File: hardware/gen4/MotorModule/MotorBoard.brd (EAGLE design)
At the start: 34 x 61.7 mm, 67 parts, among them IC1 XMEGA16A4A, M1O1 TEST_PT, M1O2 TEST_PT, M1O3 TEST_PT

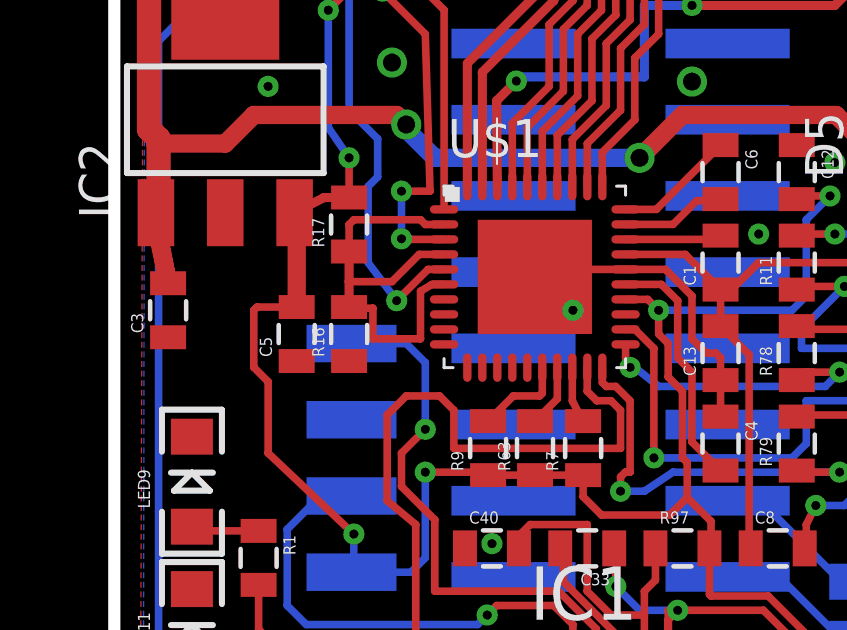
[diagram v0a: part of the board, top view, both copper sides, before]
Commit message: passes erc
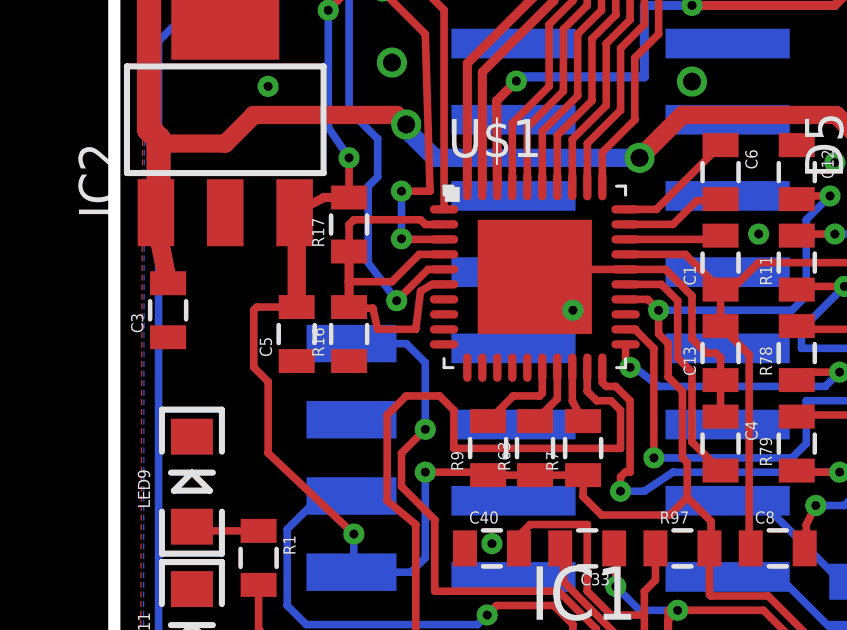
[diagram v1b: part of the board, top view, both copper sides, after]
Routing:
- net N$22: track 15.7 -> 14.8 mm
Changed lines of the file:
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@@
 <wire x1="9.9925" y1="10.06875" x2="9.5925" y2="10.06875" width="0.254" layer="1"/>
 <wire x1="9.5925" y1="10.06875" x2="9.2075" y2="9.8425" width="0.254" layer="1"/>
-<wire x1="9.2075" y1="9.8425" x2="9.2075" y2="8.255" width="0.254" layer="1"/>
-<wire x1="9.2075" y1="8.255" x2="7.62" y2="8.255" width="0.254" layer="1"/>
-<wire x1="7.62" y1="8.255" x2="7.62" y2="9.275" width="0.254" layer="1"/>
+<wire x1="9.2075" y1="9.8425" x2="9.04875" y2="8.5725" width="0.254" layer="1"/>
+<wire x1="9.04875" y1="8.5725" x2="7.77875" y2="8.5725" width="0.254" layer="1"/>
+<wire x1="7.77875" y1="8.5725" x2="7.62" y2="9.275" width="0.254" layer="1"/>
 <wire x1="9.9925" y1="12.06875" x2="9.36625" y2="12.065" width="0.254" layer="1"/>
 <wire x1="9.36625" y1="12.065" x2="9.2075" y2="12.22375" width="0.254" layer="1"/>
